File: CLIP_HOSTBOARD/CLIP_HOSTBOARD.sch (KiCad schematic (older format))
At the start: 6 parts, among them J1 505567-0671, J2 1x2_header, J3 1x5_header, U1 Buffer

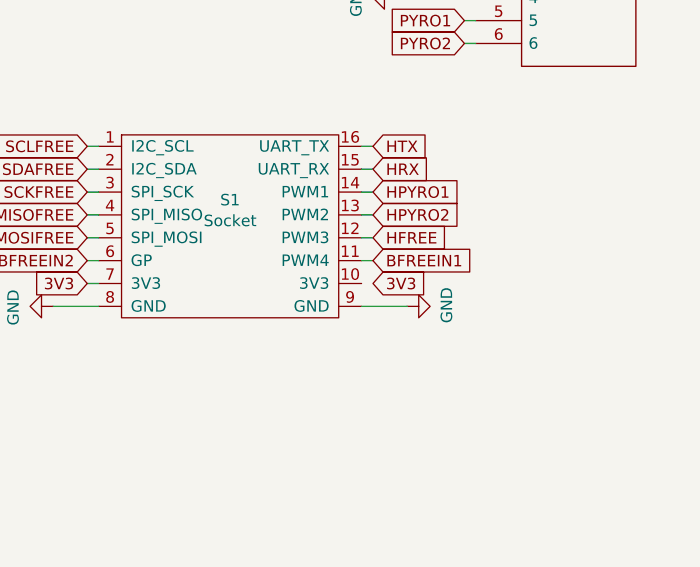
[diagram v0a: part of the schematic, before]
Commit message: duh
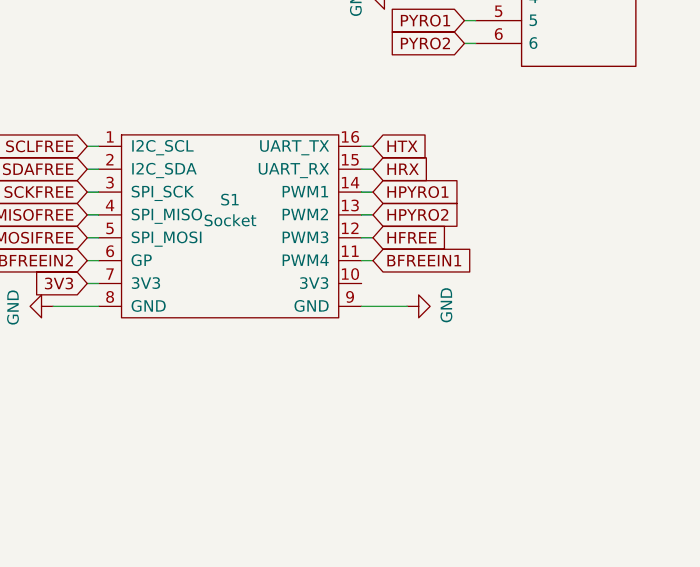
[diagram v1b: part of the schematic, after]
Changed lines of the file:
@@
 Wire Wire Line
 	6700 3050 6750 3050
-Text GLabel 6300 4400 2    50   Input ~ 0
-3V3
 Text GLabel 5050 4400 0    50   Input ~ 0
 3V3

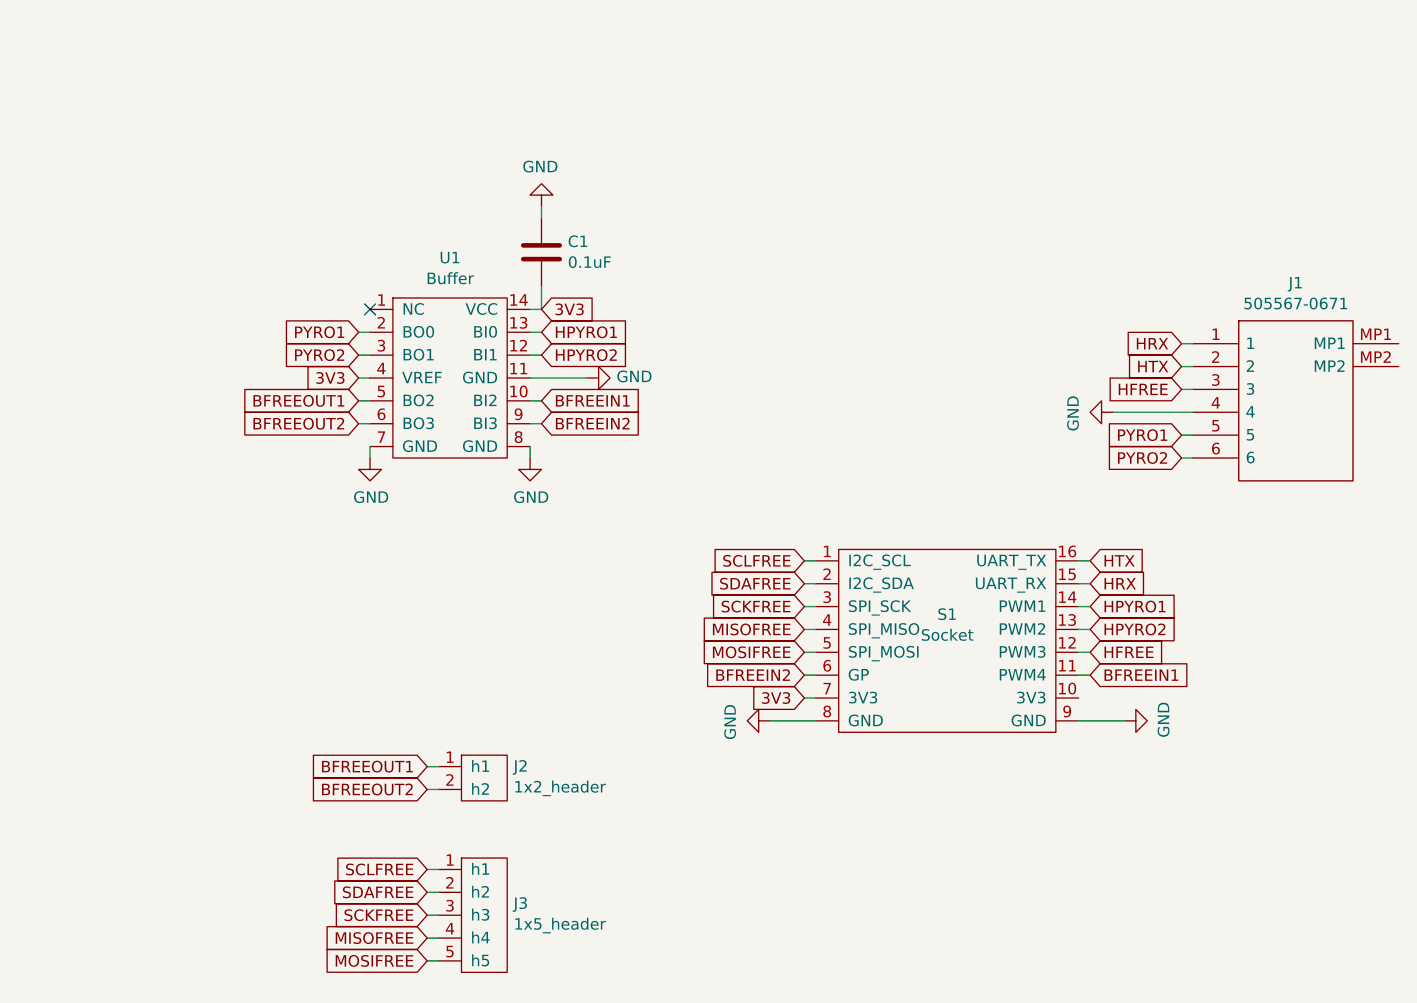
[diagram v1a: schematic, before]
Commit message: Last changes
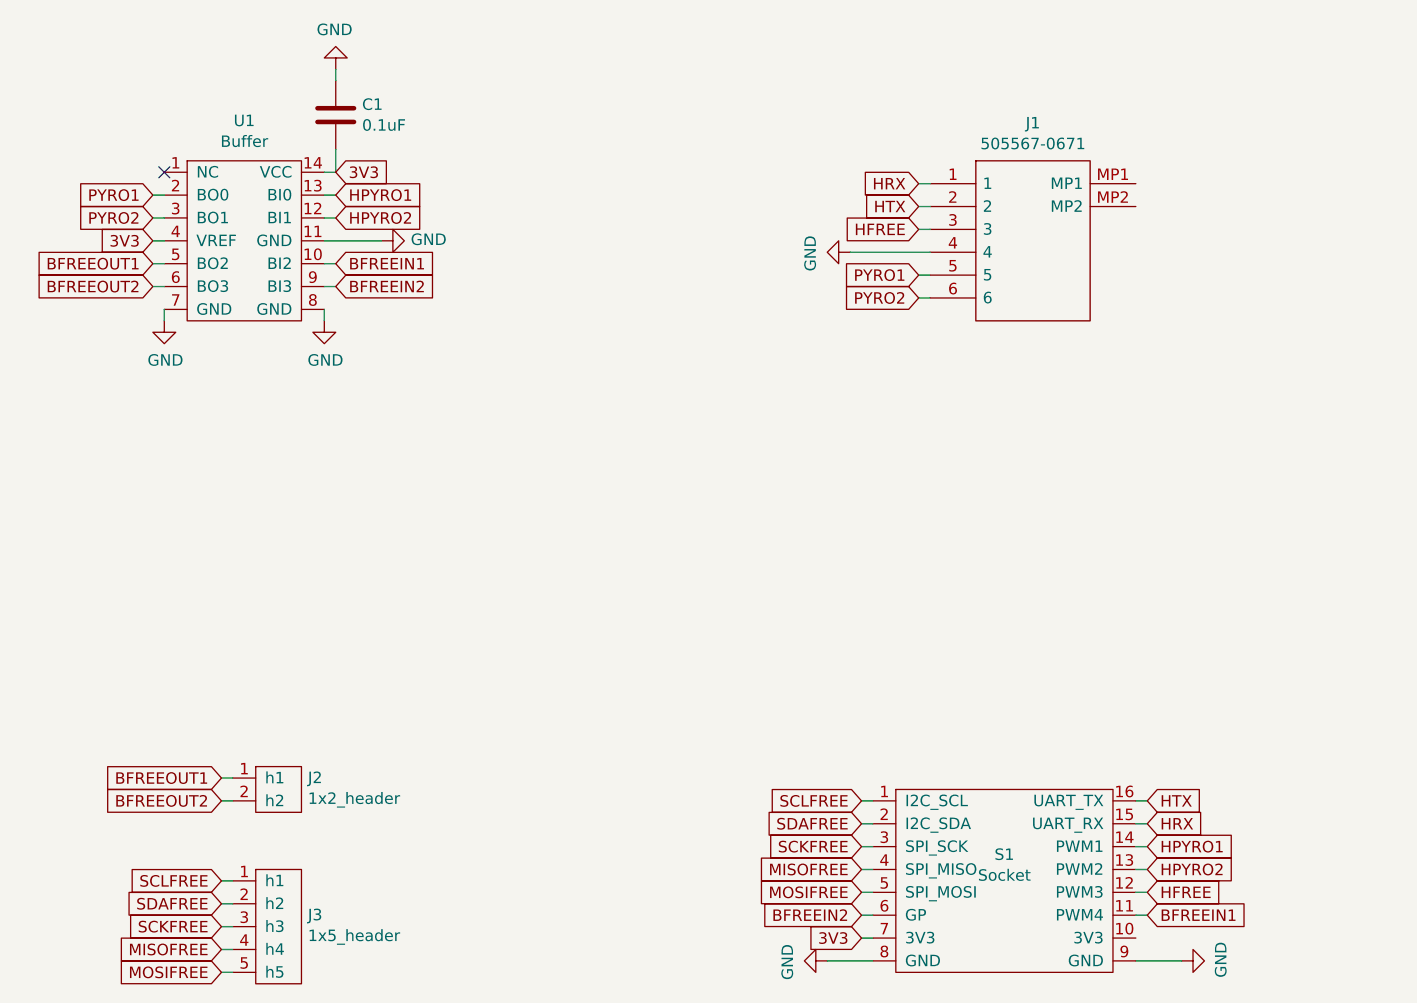
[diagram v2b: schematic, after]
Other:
- moved on the sheet: C1, J1, J2, J3, S1, U1
